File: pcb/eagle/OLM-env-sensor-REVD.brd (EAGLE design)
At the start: 47 x 30.5 mm, 7 parts, among them J1 1X2-3.5MM, U2 AM2302

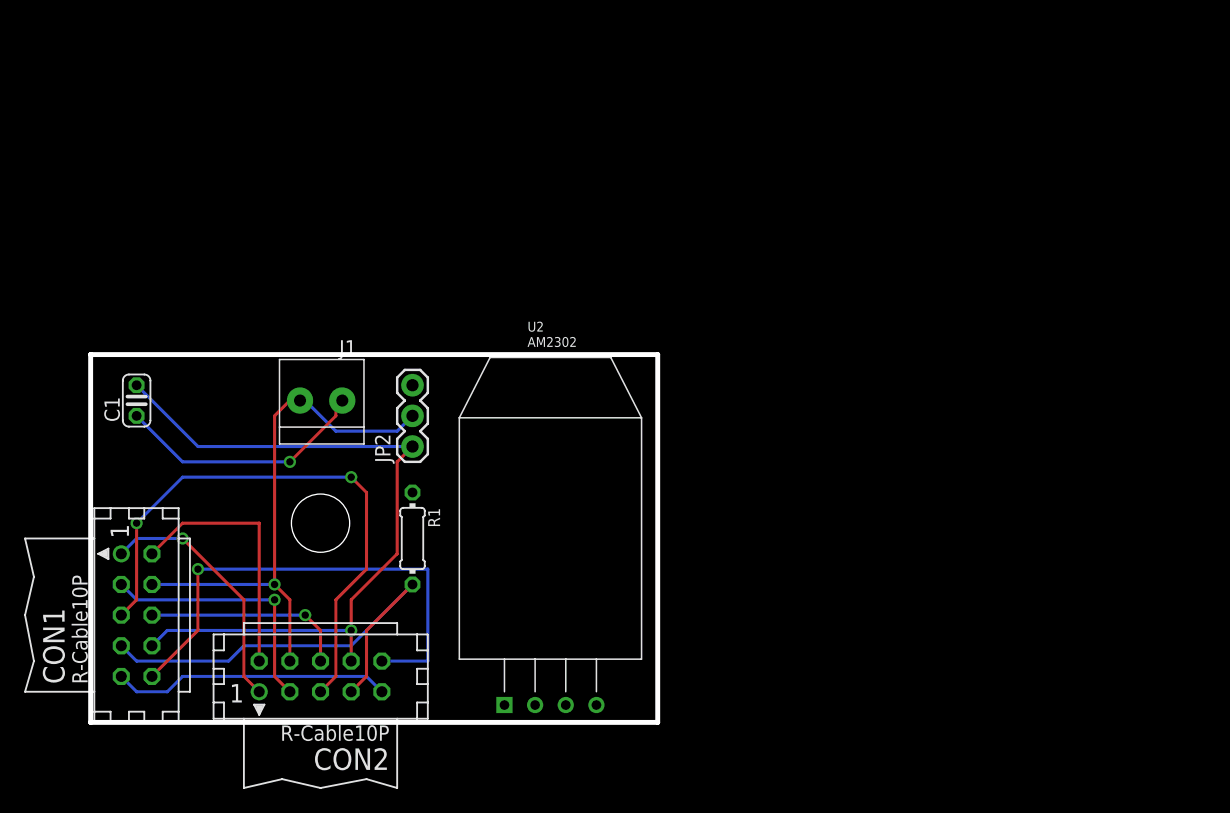
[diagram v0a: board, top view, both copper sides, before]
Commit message: edited env sensor board
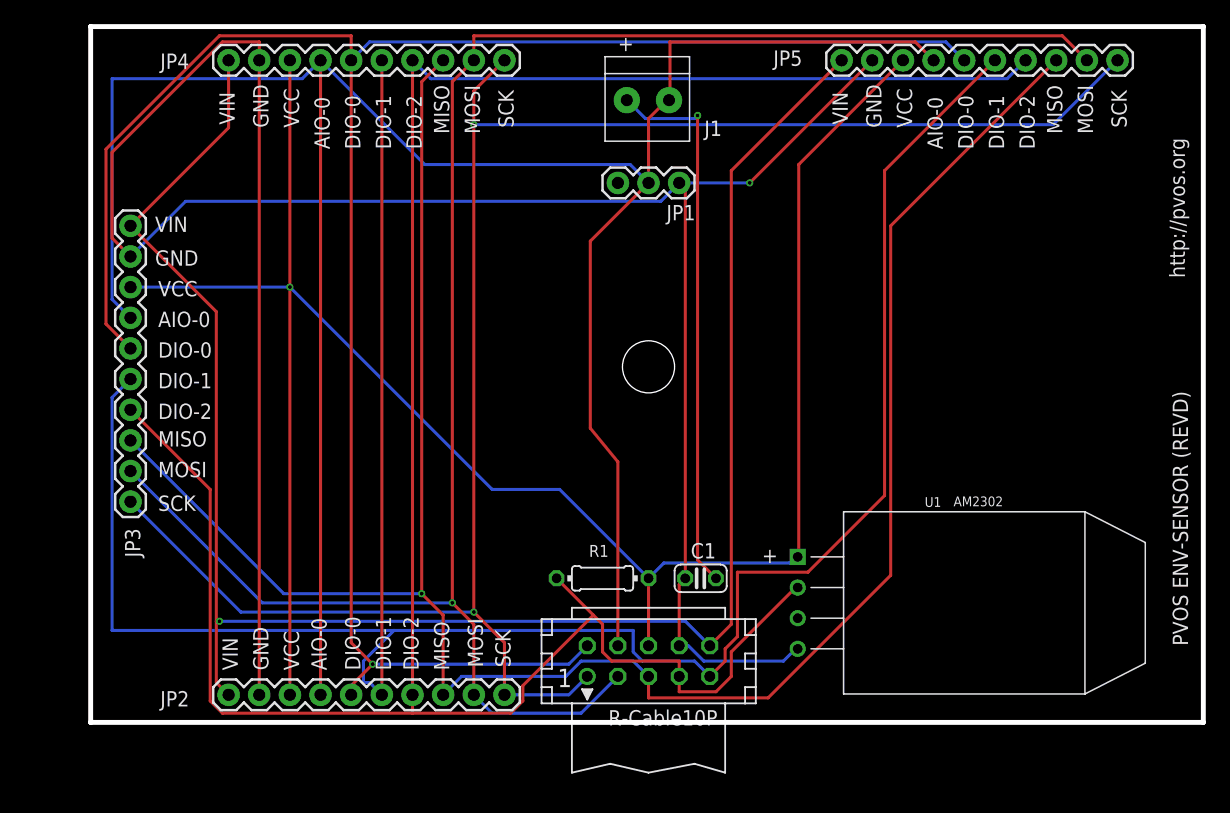
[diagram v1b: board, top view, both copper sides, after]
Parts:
- removed CON2: (no value), con-harting:CON10L
- removed U2: AM2302, sensor:AM2302
- added JP1: (no value), SparkFun-Connectors:1X03
- added JP3, JP4, JP5: M10", SparkFun-Connectors:1X10
- added U1: AM2302, sensor:AM2302
- JP2: value (none) -> M10"; device SparkFun-Connectors:1X03 -> SparkFun-Connectors:1X10
- moved C1 49.0 mm to (50.5, 11.9), turned to 180 degrees
- moved CON1 42.6 mm to (46.2, 5.08), turned to 180 degrees
- moved J1 36.9 mm to (46.2, 51.6), turned to 180 degrees
- moved JP2 25.6 mm to (11.4, 2.29), turned to 0 degrees
- moved R1 16.1 mm to (42.4, 11.9), turned to 180 degrees
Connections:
- removed net AIO: CON1.4, CON2.4, J1.2, JP2.2
- removed net DIO1: CON1.2, CON2.2
- removed net DIO2: CON1.9, CON2.9
- removed net DIO3: CON1.7, CON2.7, R1.2, U2.P$2
- removed net VDD: R1.1, U2.P$1
- new net AIO-0: CON1.4, J1.2, JP1.2, JP2.4, JP3.4, JP4.4, JP5.4
- new net DIO-0: CON1.2, JP2.5, JP3.5, JP4.5, JP5.5
- new net DIO-1: CON1.9, JP2.6, JP3.6, JP4.6, JP5.6
- new net DIO-2: CON1.7, JP2.7, JP3.7, JP4.7, JP5.7, R1.2, U1.P$2
- net GND: now also JP1.1, JP2.2, JP3.2, JP4.2, JP5.2, U1.P$4; no longer CON2.8, JP2.1, U2.P$4
- net MISO: now also JP2.8, JP3.8, JP4.8, JP5.8; no longer CON2.5
- net MOSI: now also JP2.9, JP3.9, JP4.9, JP5.9; no longer CON2.3
- net SCK: now also JP2.10, JP3.10, JP4.10, JP5.10; no longer CON2.1
- net VCC: now also JP2.3, JP3.3, JP4.3, JP5.3, R1.1, U1.P$1; no longer CON2.6
- net VIN: now also JP2.1, JP3.1, JP4.1, JP5.1; no longer CON2.10
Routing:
- net DIO-2: track 0.00 -> 200.8 mm
- net AIO-0: track 0.00 -> 198.5 mm
- net DIO-1: track 0.00 -> 197.8 mm
- net DIO-0: track 0.00 -> 168.1 mm, vias 0 -> 1
- net VCC: track 17.0 -> 169.0 mm
- net GND: track 61.9 -> 197.1 mm
- net MOSI: track 21.4 -> 152.8 mm
- net MISO: track 47.4 -> 176.5 mm, vias 2 -> 1
- net SCK: track 20.9 -> 150.0 mm, vias 1 -> 2
- net VIN: track 40.9 -> 154.1 mm
- net AIO: track 44.5 -> 0.00 mm, vias 1 -> 0
- net DIO3: track 38.3 -> 0.00 mm
- net 3.3V: track 21.5 -> 45.6 mm
- net DIO2: track 23.2 -> 0.00 mm
- net DIO1: track 21.4 -> 0.00 mm
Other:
- board size 47 x 30.5 mm -> 92.2 x 57.7 mm
- board text added: "+"
- board text added: "AIO-0"
- board text added: "DIO-0"
- board text added: "DIO-1"
- board text added: "DIO-2"
- board text added: "GND"
- board text added: "MISO"
- board text added: "MOSI"
- board text added: "PVOS ENV-SENSOR (REVD)"
- board text added: "SCK"
- board text added: "VCC"
- board text added: "VIN"
- board text added: "http://pvos.org"
